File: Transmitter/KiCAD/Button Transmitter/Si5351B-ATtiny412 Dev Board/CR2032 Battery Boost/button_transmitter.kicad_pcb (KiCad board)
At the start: 2 copper layers, 24.4 x 24.4 mm, 35 parts, among them J1 1.27mm Pogo Pads, J2 Conn_Coaxial, Q1 MMUN2238LT1G, U1 ATtiny412-SS, U2 Si5351B-B-GM1, U3 TLV61070ADBV, Y1 25MHz

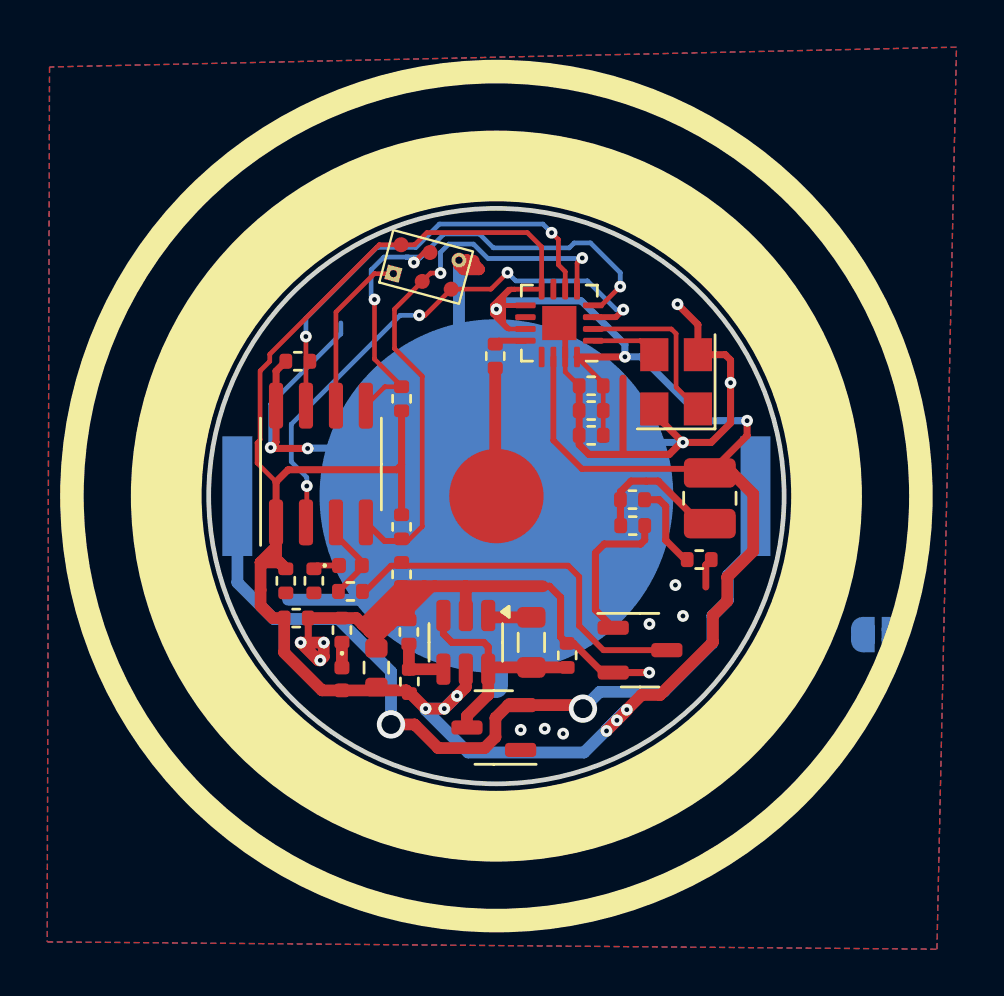
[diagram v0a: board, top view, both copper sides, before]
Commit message: Finished CR2032 PCB layout
I like this. This is good
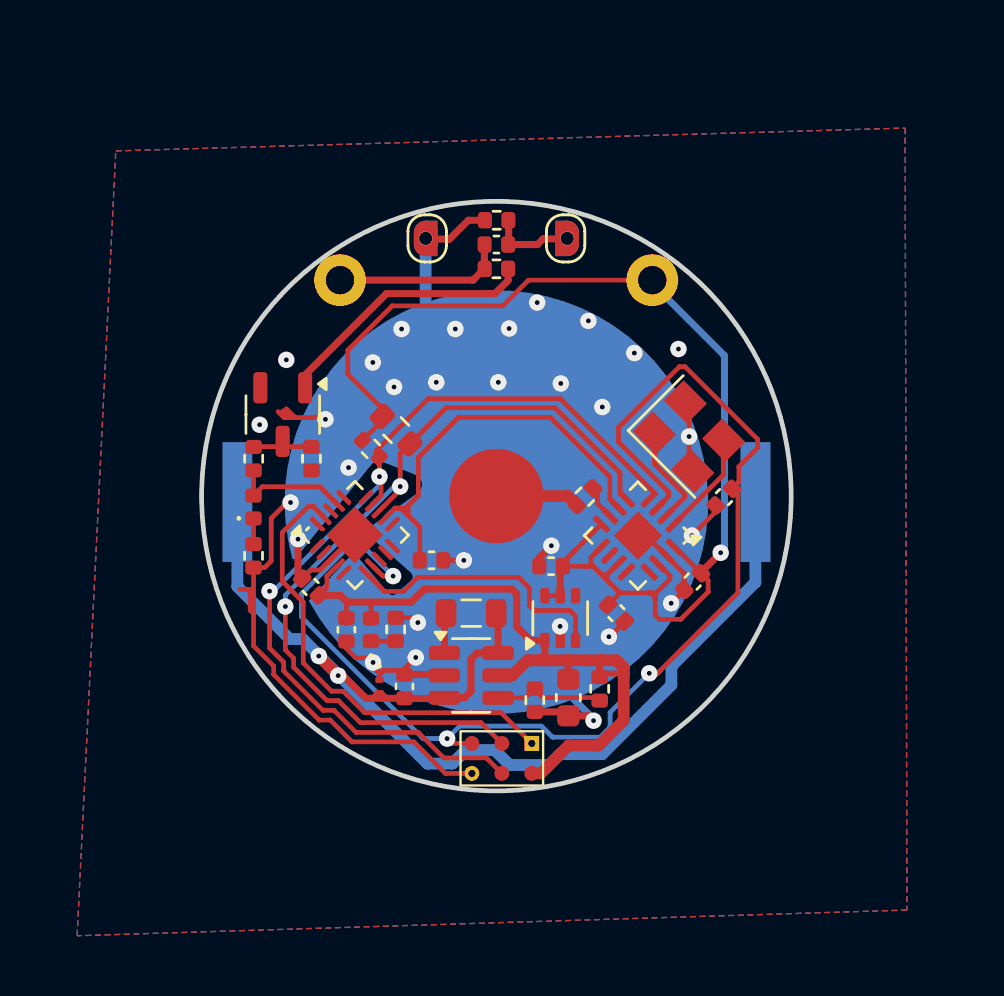
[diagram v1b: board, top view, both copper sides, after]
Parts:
- removed the J1 at (72.6, 94.2)
- added BZ2-1: 7BB-20-3, Library:Buzzer_Pad_NEG, B.Cu at (72.6, 93.0)
- added C8: 100nF, Library:Worthington_C_0402_1005Metric, F.Cu at (72.9, 106.6)
- added J2: 1.27mm Pogo Pads For Programming & Debug, Library:2x3_1.27mm_Pogo_Header, F.Cu at (75.8, 115.0)
- added U5: TLV61070ADBV, Package_TO_SOT_SMD:SOT-23-6, F.Cu at (74.6, 111.5)
- BT1: footprint Battery:BatteryHolder_Keystone_3034_1x20mm -> Library:BatteryHolder_Keystone_3034_1x20mm_CUTOUT
- BZ1: value Buzzer Pads -> 7BB-20-3; footprint Jumper:SolderJumper-2_P1.3mm_Open_RoundedPad1.0x1.5mm -> Library:Buzzer_Pad_POS
- C1, C4, C5, C6, C7: footprint Resistor_SMD:R_0402_1005Metric -> Library:Worthington_C_0402_1005Metric
- C10: value 10uF -> 22uF; footprint Resistor_SMD:R_0402_1005Metric -> Capacitor_SMD:C_0603_1608Metric
- C2: value 10uF -> 100nF; footprint Resistor_SMD:R_0402_1005Metric -> Library:Worthington_C_0402_1005Metric
- C3: value 100nF -> 10uF; footprint Resistor_SMD:R_0402_1005Metric -> Library:Worthington_C_0402_1005Metric
- C9: value 22uF -> 10uF; footprint Resistor_SMD:R_0603_1608Metric -> Library:Worthington_C_0402_1005Metric
- D1, D3: footprint LED_SMD:LED_0402_1005Metric -> Library:Worthington_LED_0402_1005Metric
- D2: value LS0504EVT233 -> ESD156B1W; footprint Package_TO_SOT_SMD:SOT-23-3 -> Diode_SMD:D_0201_0603Metric
- J1: renamed from J2; value Conn_Coaxial -> Antenna Screw Pad
- L1: value 220uH -> 100mH; footprint Inductor_SMD:L_1008_2520Metric -> Inductor_THT:L_Axial_L12.0mm_D5.0mm_P15.24mm_Horizontal_Fastron_MISC
- R1: value 1k8 -> 10k; footprint Resistor_SMD:R_0402_1005Metric -> Library:Worthington_R_0402_1005Metric
- R10, R11, R5, R6, R7, R9: footprint Resistor_SMD:R_0402_1005Metric -> Library:Worthington_R_0402_1005Metric
- R3: value 0R -> 1k8; footprint Resistor_SMD:R_0402_1005Metric -> Resistor_SMD:R_0603_1608Metric
- R4: value 10k -> 0R; footprint Resistor_SMD:R_0402_1005Metric -> Library:Worthington_R_0402_1005Metric
- R8: value 100 -> 220; footprint Resistor_SMD:R_0402_1005Metric -> Library:Worthington_R_0402_1005Metric
- U1: value ATtiny412-SS -> TPS22919DCK; footprint Package_SO:SOIC-8_3.9x4.9mm_P1.27mm -> Package_TO_SOT_SMD:SOT-363_SC-70-6
- U3: value TLV61070ADBV -> ATtiny416-M; footprint Package_TO_SOT_SMD:SOT-23-6 -> Package_DFN_QFN:VQFN-20-1EP_3x3mm_P0.4mm_EP1.7x1.7mm
- U4: value ~ -> Case
- moved BZ1 21.4 mm to (78.6, 93.0), turned to 180 degrees
- moved L1 18.6 mm to (68.0, 95.8), turned to 0 degrees
- moved Q1 18.1 mm to (66.6, 100.5), turned to -90 degrees
- moved C1 17.3 mm to (83.9, 107.5), turned to -135 degrees
- moved C5 14.7 mm to (69.3, 109.6), turned to -90 degrees
- moved C4 14.1 mm to (67.7, 107.8), turned to 135 degrees
- moved R1 13.6 mm to (75.6, 92.2), turned to 180 degrees
- moved R5 12.3 mm to (75.6, 94.3)
- moved U1 12.1 mm to (78.3, 109.1)
- moved C2 11.0 mm to (77.9, 106.9), turned to 180 degrees
- moved C6 9.77 mm to (75.6, 93.2)
- moved U2 9.61 mm to (81.6, 105.6), turned to -135 degrees
- moved R9 8.08 mm to (80.0, 112.1), turned to -90 degrees
- moved C3 7.62 mm to (80.7, 108.9), turned to -45 degrees
- moved R6 6.97 mm to (65.3, 102.3), turned to 90 degrees
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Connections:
- C1 pad 1: +3V3 -> /+3V3_SW
- C10 pad 1: Net-(D2-OUT) -> +3V3
- C2 pad 1: +3V3 -> /+3V3_SW
- C3 pad 1: +3V3 -> /+3V3_SW
- C6 pad 1: GND -> Net-(C6-Pad1)
- C6 pad 2: /~{TX_EN} -> Net-(BZ1-+)
- C7 pad 1: Net-(C7-Pad1) -> GND
- C7 pad 2: Net-(BZ1-+) -> /MCU_DAC0
- C9 pad 1: +3V3 -> Net-(BT1-+)
- D1 pad 2: Net-(D1-A) -> /BUZZER_PULSE
- J1 pad 1: /CLK3 -> /CLK1
- L1 pad 1: Net-(C7-Pad1) -> Net-(C6-Pad1)
- L1 pad 2: +3V3 -> /+3V3_SW
- L2 pad 1: Net-(D2-OUT) -> Net-(BT1-+)
- L2 pad 2: Net-(U3-SW) -> Net-(U5-SW)
- R1 pad 1: +3V3 -> Net-(BZ1-+)
- R1 pad 2: /MCU_SDA -> GND
- R10 pad 1: Net-(U3-V_{FB}) -> Net-(U5-V_{FB})
- R2 pad 1: +3V3 -> /+3V3_SW
- R3 pad 1: /CLK3_T -> /+3V3_SW
- R3 pad 2: /CLK3 -> /MCU_SDA
- R4 pad 1: Net-(BZ1-+) -> /CLK1_T
- R4 pad 2: GND -> /CLK1
- R5 pad 2: Net-(C7-Pad1) -> Net-(C6-Pad1)
- R6 pad 1: Net-(D1-A) -> /BUZZER_PULSE
- R9 pad 2: Net-(U3-V_{FB}) -> Net-(U5-V_{FB})
- U1 pad 2: /MCU_DAC0 -> GND
- U1 pad 3: Net-(D1-A) -> /OUTPUT_PWR_EN
- U1 pad 4: /MCU_SDA -> (no net)
- U1 pad 5: /MCU_SCL -> /+3V3_SW
- U1 pad 6: /MCU_UPDI -> /+3V3_SW
- U2 pad 11: +3V3 -> /+3V3_SW
- U2 pad 12: /CLK3_T -> unconnected-(U2-CLK3-Pad12)
- U2 pad 14: +3V3 -> /+3V3_SW
- U2 pad 16: +3V3 -> /+3V3_SW
- U2 pad 7: unconnected-(U2-CLK1-Pad7) -> /CLK1_T
- U2 pad 8: +3V3 -> /+3V3_SW
- U2 pad 9: +3V3 -> /+3V3_SW
- U3 pad 1: Net-(U3-SW) -> unconnected-(U3-PA2-Pad1)
- U3 pad 2: GND -> unconnected-(U3-PA3-Pad2)
- U3 pad 3: Net-(D2-OUT) -> GND
- U3 pad 4: Net-(U3-V_{FB}) -> +3V3
- U3 pad 5: +3V3 -> unconnected-(U3-PA4-Pad5)
- U3 pad 6: Net-(D2-OUT) -> /OUTPUT_PWR_EN
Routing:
- net +3V3: track 122.8 -> 31.2 mm, vias 9 -> 0
- net /+3V3_SW: track 0.00 -> 53.9 mm, vias 0 -> 1
- net GND: track 125.6 -> 77.7 mm, vias 15 -> 30
- net /MCU_DAC0: track 23.3 -> 52.9 mm, vias 4 -> 3
- net /MCU_SCL: track 23.7 -> 38.9 mm, vias 3 -> 2
- net Net-(Q1-G): track 16.1 -> 2.63 mm
- net /MCU_UPDI: track 7.67 -> 19.4 mm
- net /OUTPUT_PWR_EN: track 0.00 -> 11.6 mm
- net /MCU_SDA: track 24.0 -> 35.4 mm
- net Net-(BT1-+): track 37.5 -> 48.9 mm
- net Net-(D2-OUT): track 10.1 -> 0.00 mm
- net Net-(C6-Pad1): track 0.00 -> 7.35 mm
- net Net-(C7-Pad1): track 5.78 -> 0.00 mm
- net /CLK3: track 5.46 -> 0.00 mm
- net /BUZZER_PULSE: track 0.00 -> 5.11 mm
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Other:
- board size 24.4 x 24.4 mm -> 25 x 25 mm
